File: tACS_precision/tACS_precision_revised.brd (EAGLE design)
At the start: 49.2 x 49.5 mm, 48 parts, among them IC1 TLC2252, IC2 LM4040, IC3 TLC2252, IC4 LM4040, IC5 ADR5041, IC6 REF5050AIDR, IC7 78L05ACD, T1 FMMT734, T2 FMMT634, T3 FMMT634, T4 FMMT734, T5 FMMT734, T6 FMMT634

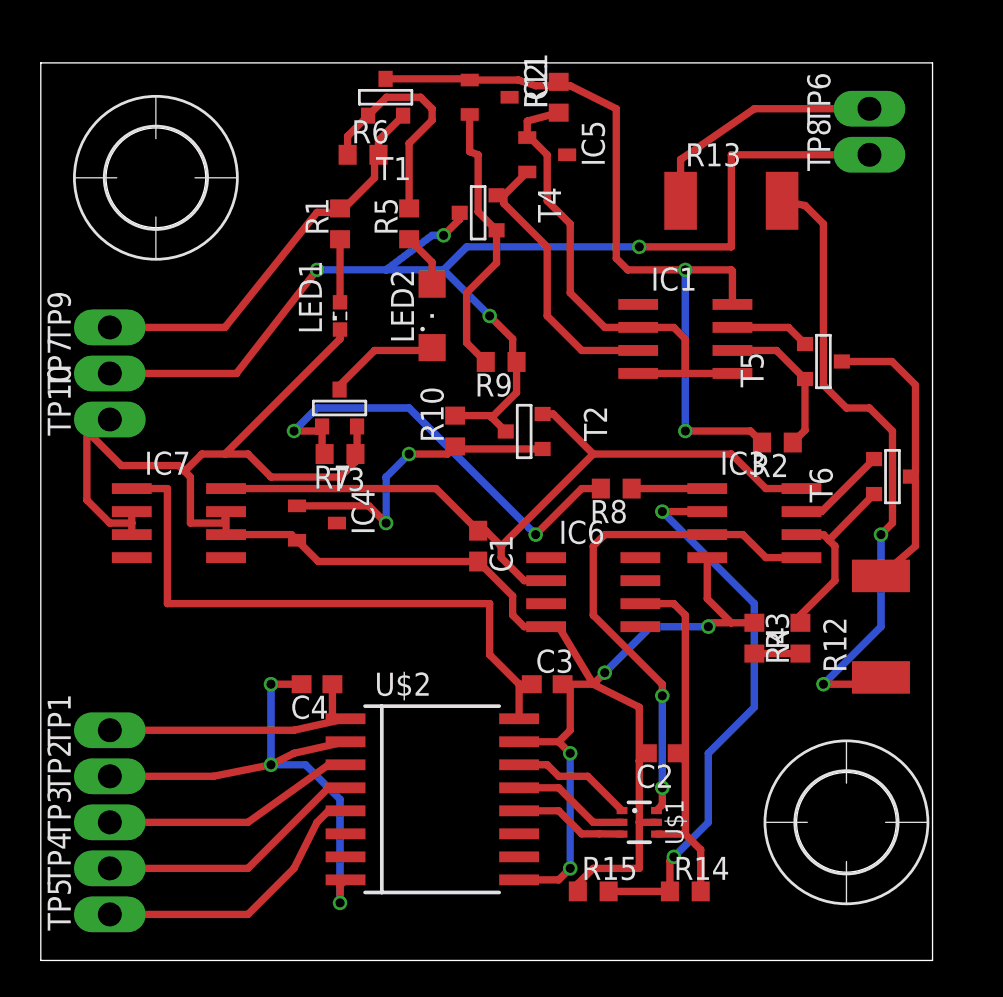
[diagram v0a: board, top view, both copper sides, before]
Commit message: including revised board files
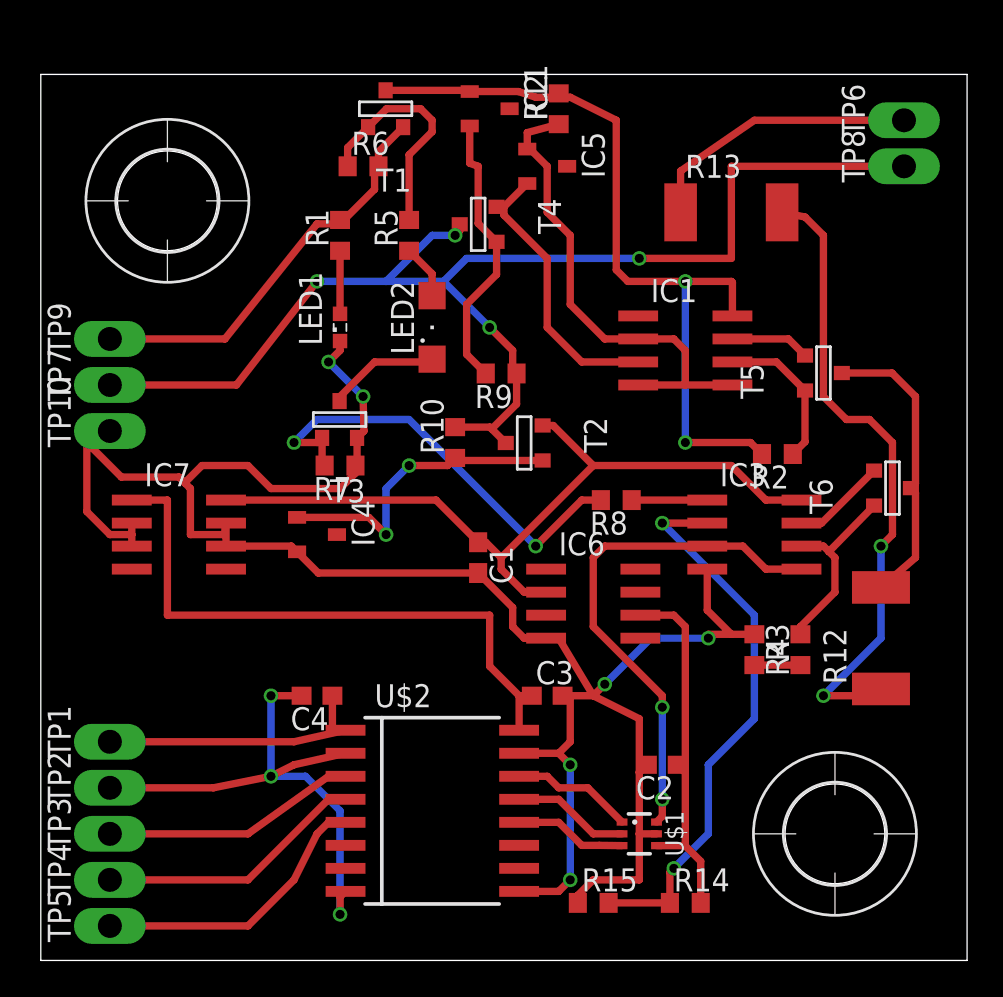
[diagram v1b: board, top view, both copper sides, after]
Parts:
- IC7: value 78L05ACD -> L78L05
- moved TP6 2.01 mm to (47.6, 46.4)
- moved TP8 2.01 mm to (47.6, 43.8)
- moved H2 1.42 mm to (6.99, 41.9)
- moved H1 0.90 mm to (43.8, 6.99)
- moved IC5 0.64 mm to (27.9, 43.8)
- moved LED1 0.64 mm to (16.5, 34.9)
- moved LED2 0.64 mm to (21.6, 34.9)
- moved R6 0.64 mm to (17.8, 43.8)
- moved R9 0.64 mm to (25.4, 32.4)
- moved T5 0.64 mm to (43.2, 32.4)
- moved IC6 0.64 mm to (30.5, 19.7)
- moved R10 0.64 mm to (22.9, 28.6)
- moved R3 0.64 mm to (41.9, 17.1)
- moved R4 0.64 mm to (39.4, 17.1)
- moved R7 0.64 mm to (16.5, 27.3)
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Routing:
- net N$3: track 119.8 -> 116.9 mm, vias 4 -> 6
- net N$11: track 69.3 -> 71.3 mm
- net N$24: track 13.6 -> 15.5 mm
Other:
- board size 49.2 x 49.5 mm -> 51.1 x 48.9 mm
- board text added: "ELECTRICAL ISOLATION"
- board text removed: "- ELECTRICAL ISOLATION -"
